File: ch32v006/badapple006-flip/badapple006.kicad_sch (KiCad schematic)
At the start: 31 parts, among them J1 OLED, J10 SCL, J11 SDA, J2 USB_C_Receptacle_USB2.0, J3 PG, J4 3v3, J5 GND, J6 RFO, J7 RFA, J8 APPLE, J9 RFO2, U1 CH32V006F8U6, U2 XC6206P332, Y1 24MHz

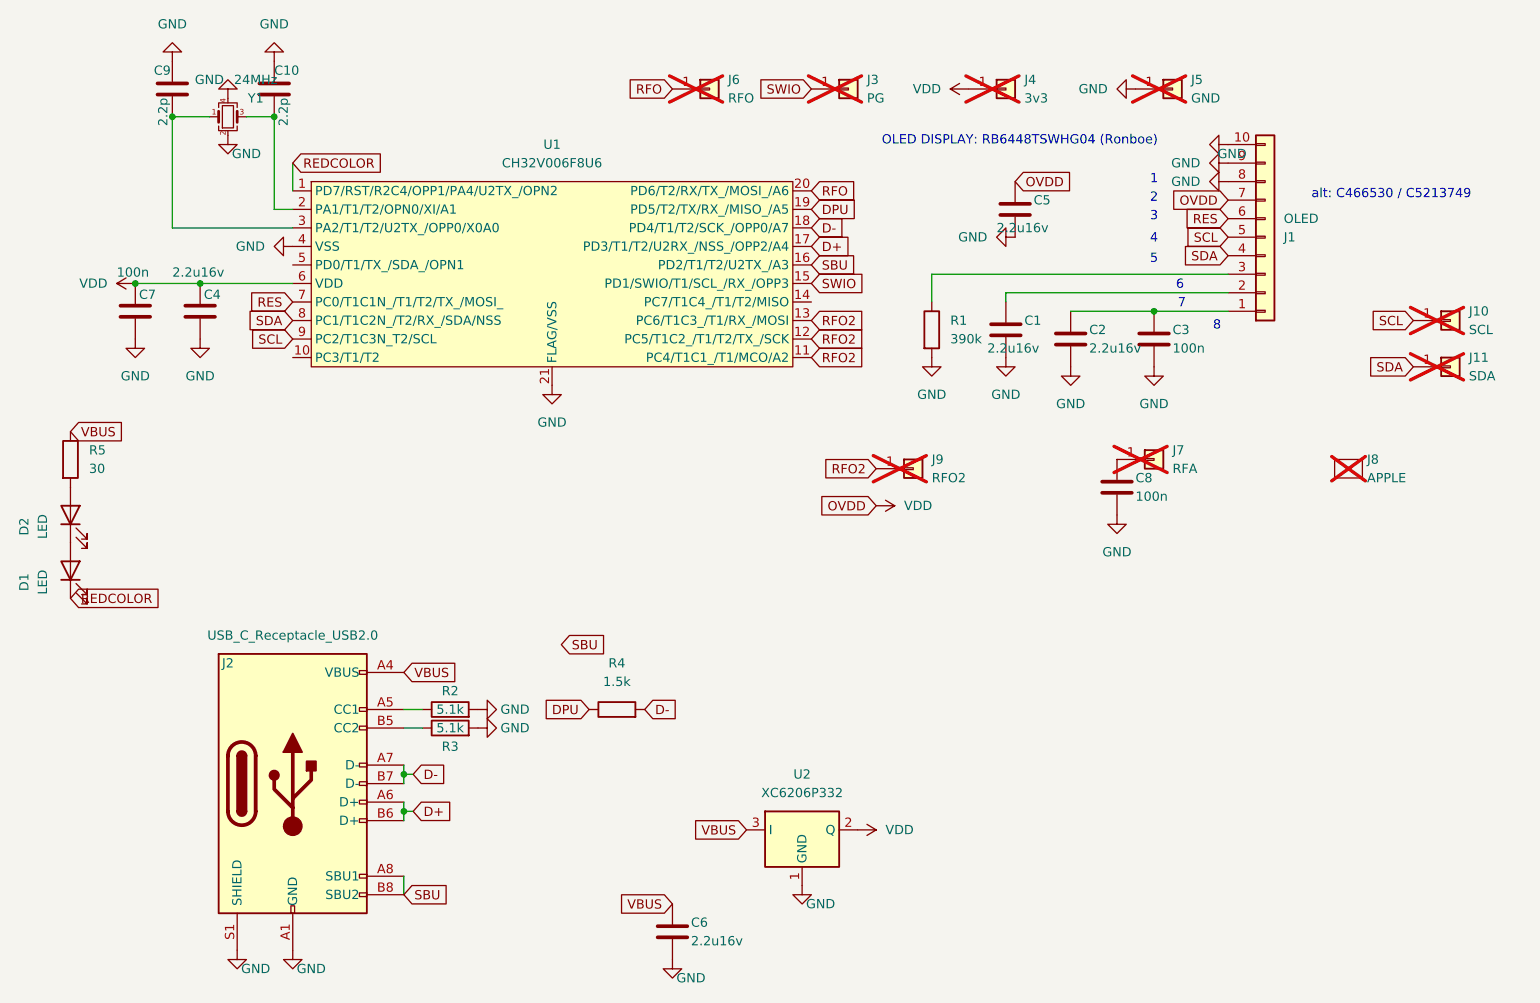
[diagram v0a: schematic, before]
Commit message: Update flip design.
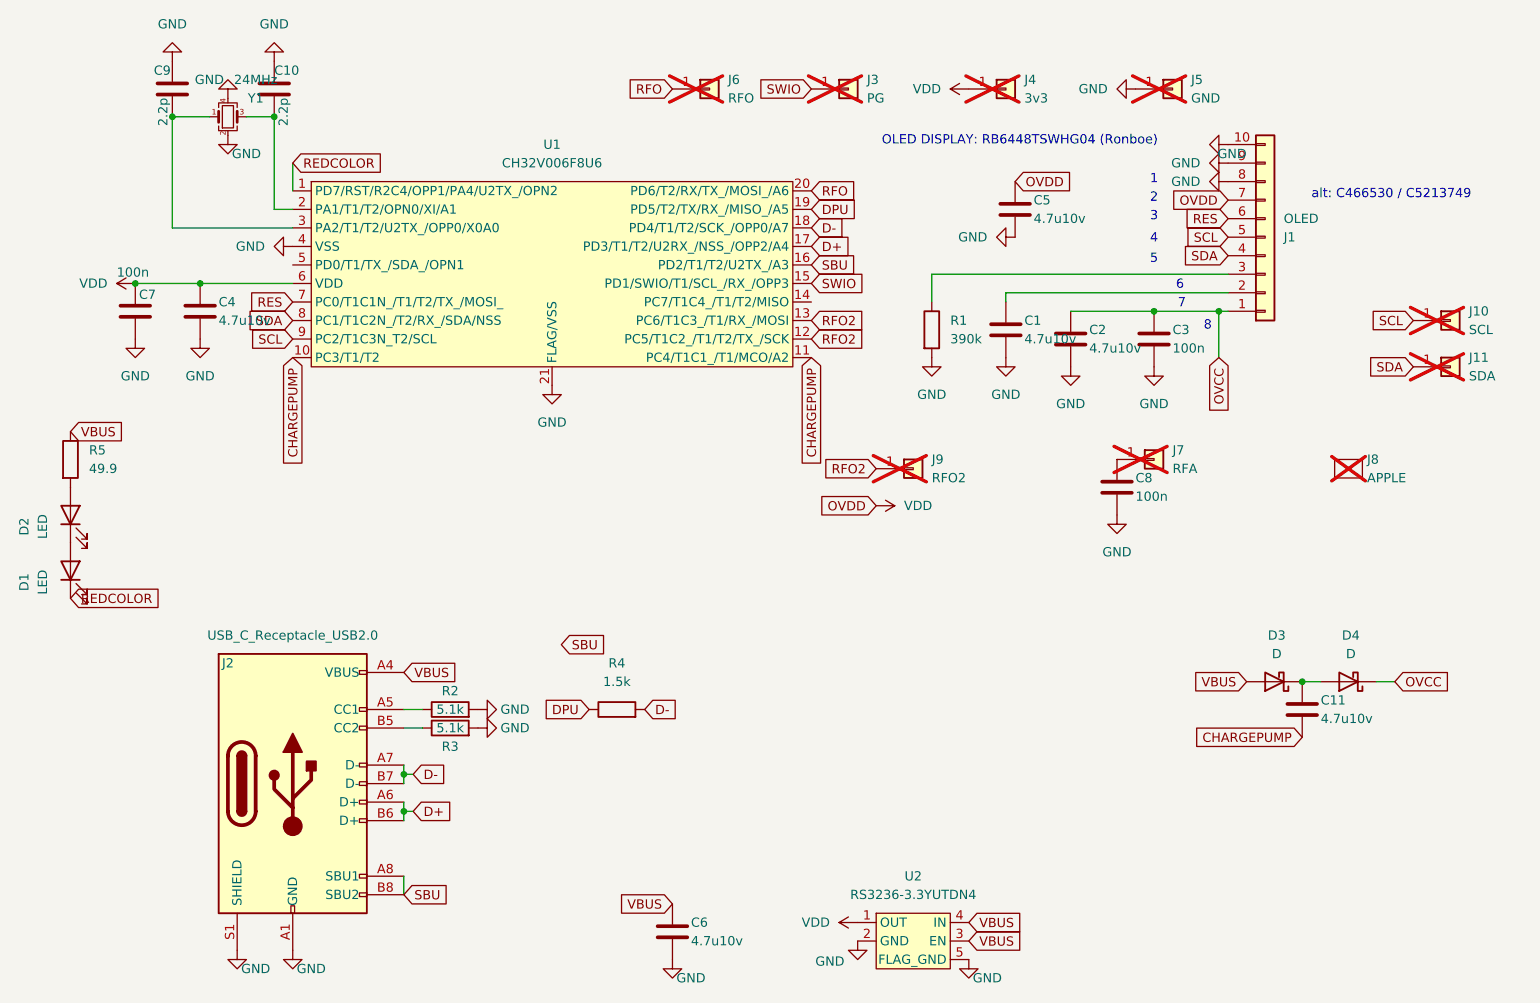
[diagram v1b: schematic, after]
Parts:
- removed U2: XC6206P332, Package_TO_SOT_SMD:SOT-23, symbol Regulator_Linear:IFX27001TFV26
- added C11: 4.7u10v, Capacitor_SMD:C_0402_1005Metric, symbol Device:C
- added D3, D4: D, Diode_SMD:D_SOD-323, symbol Device:D_Schottky
- added U2: RS3236-3.3YUTDN4, cnhardware:xdfn-reg, symbol cnhardware:RS3236-DFN-LDO
- C1, C2, C4, C5, C6: value 2.2u16v -> 4.7u10v; footprint Capacitor_SMD:C_0603_1608Metric -> Capacitor_SMD:C_0402_1005Metric; LCSC C23630 -> C23733
- R5: value 30 -> 49.9; LCSC C1091 -> C25120; now in the parts list
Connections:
- net GND: now also U2.2 (GND), U2.5 (FLAG_GND)
- net RFO2: no longer U1.11 (PC4/T1C1_/T1/MCO/A2)
- net VBUS: now also D3.2 (A), U2.3 (EN), U2.4 (IN)
- net VDD: now also U2.1 (OUT)
- net OVCC: now reaches C2.1, C3.1, J1.1 (Pin_1)
- net OVCC: now also D4.1 (K)
- net CHARGEPUMP: now reaches U1.10 (PC3/T1/T2)
- net CHARGEPUMP: now also U1.11 (PC4/T1C1_/T1/MCO/A2), C11.2
- new net: C11.1, D3.1 (K), D4.2 (A)
